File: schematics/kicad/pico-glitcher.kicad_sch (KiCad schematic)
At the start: 72 parts, among them Q1 IRLML2502, Q2 IRF7807PBF, Q3 TPS 79318, Q4 TPS2041, U1 NH245, U2 NH245, X1 BU-SMA-V, X2 BU-SMA, X3 M08X2

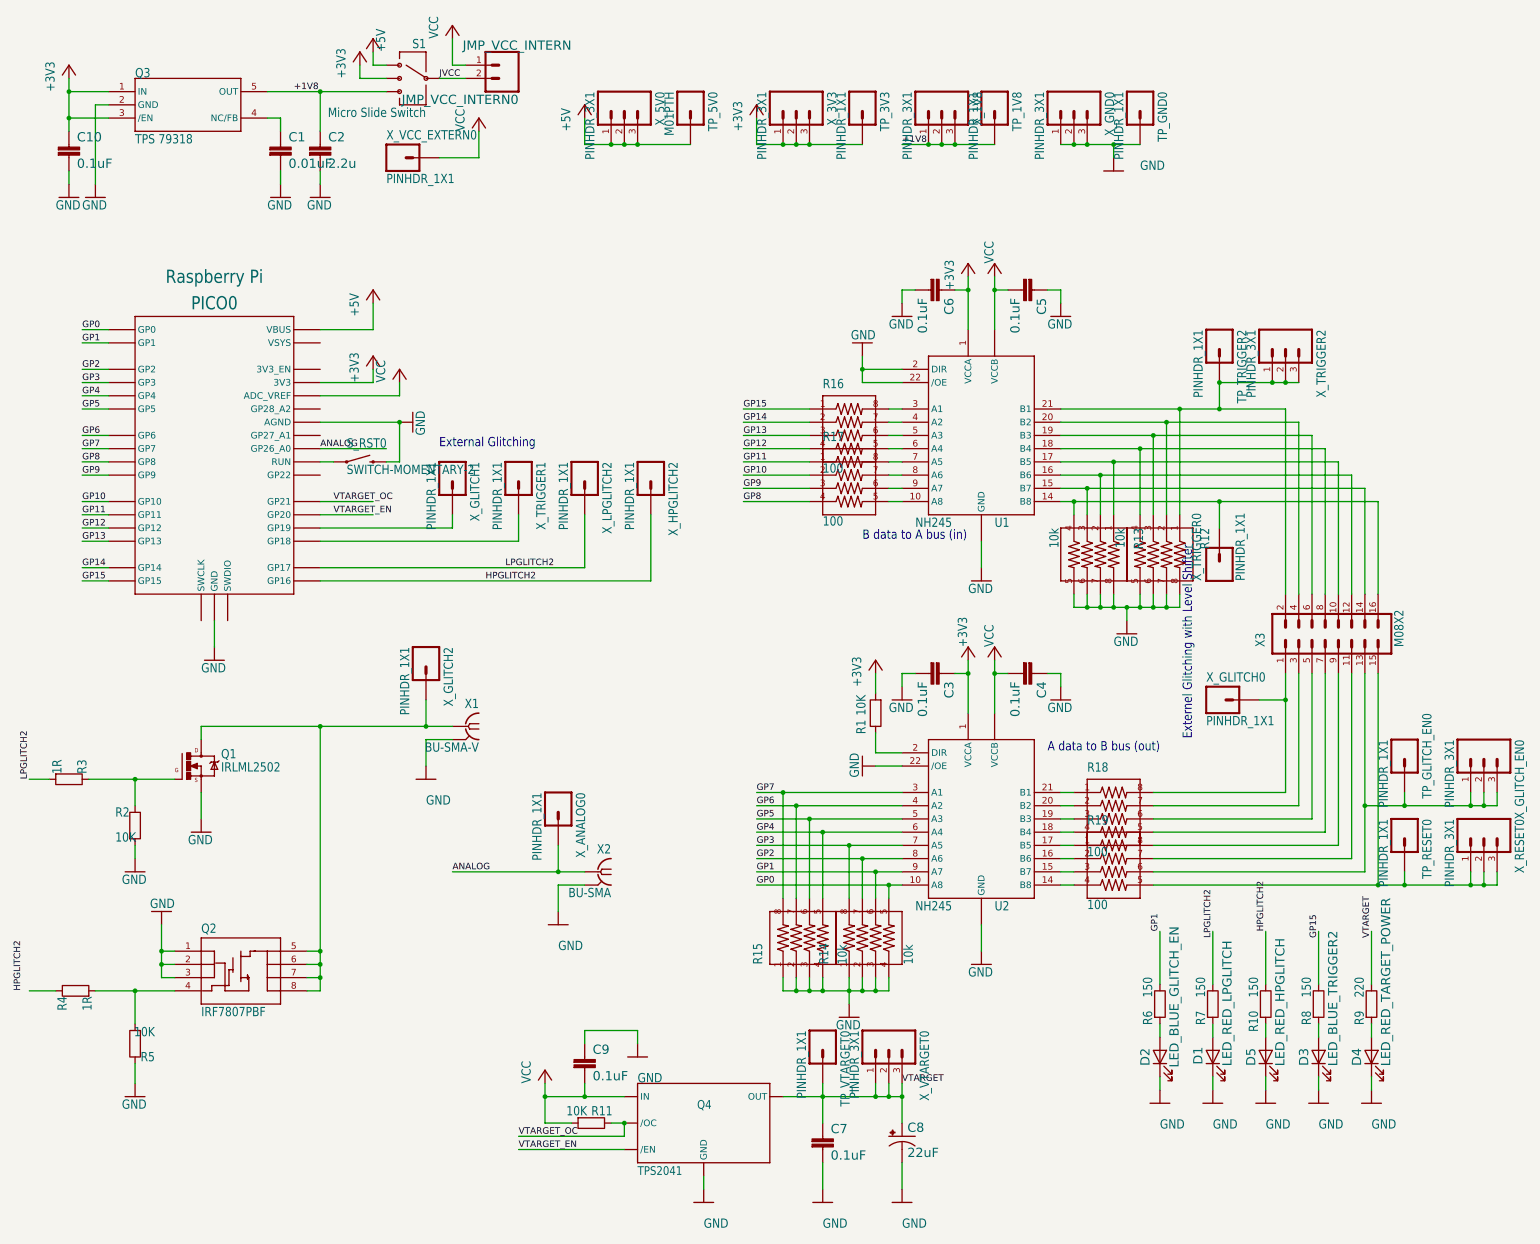
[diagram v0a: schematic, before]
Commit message: replaced 0603 capacitor's symbol and footprint with kicad library's ones
  also: simplified some tracks.
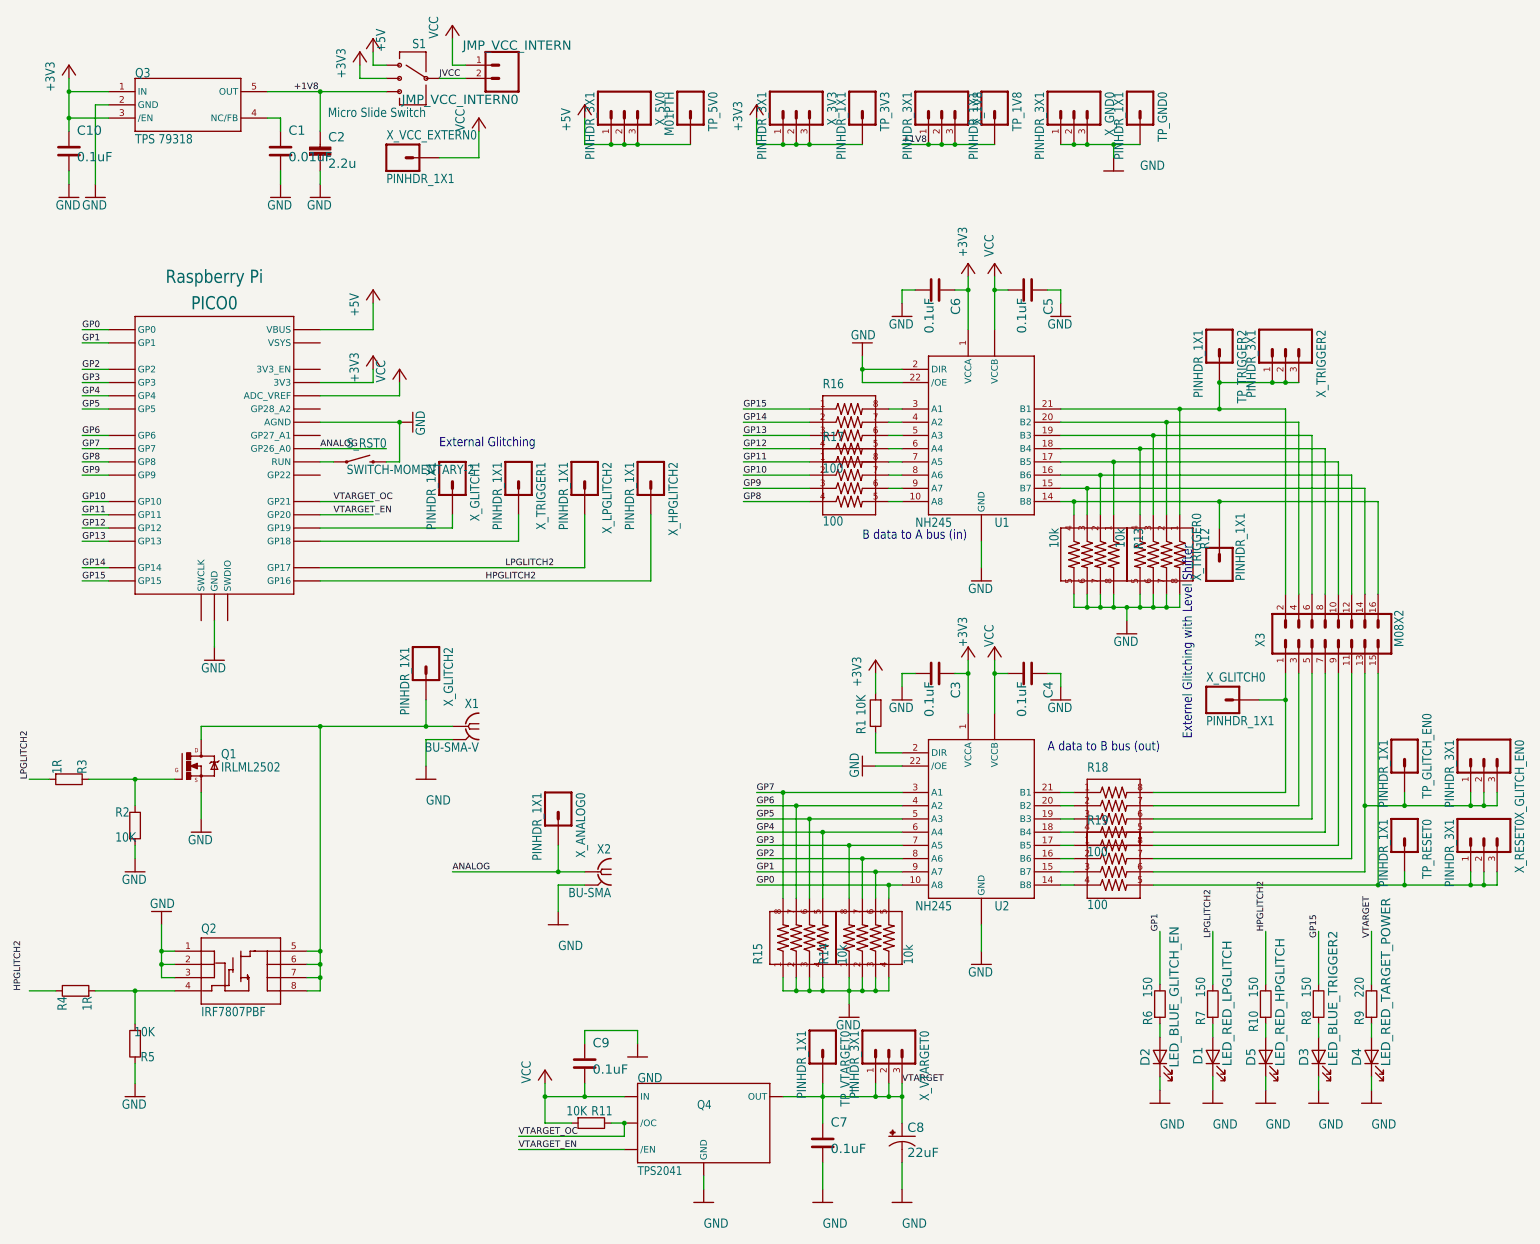
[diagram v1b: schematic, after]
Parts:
- C1, C10, C3, C4, C5, C6, C7, C9: footprint pico-glitcher:0603 -> Capacitor_SMD:C_0603_1608Metric; symbol pico-glitcher:0.1UF-0603-25V-10%-X7R-WE -> Device:C
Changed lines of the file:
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@@
 	)
 	(symbol
-		(lib_id "pico-glitcher:0.1UF-0603-25V-10%-X7R-WE")
-		(at 208.28 71.12 270)
+		(lib_id "Device:C")
+		(at 209.55 71.12 270)
 		(unit 1)
 		(exclude_from_sim no)
@@
 		(dnp no)
 		(property "Reference" "C5"
-			(at 211.201 72.644 0)
+			(at 212.471 72.644 0)
 			(effects
 				(font
@@
 		)
 		(property "Value" "0.1uF"
-			(at 206.121 72.644 0)
+			(at 207.391 72.644 0)
 			(effects
 				(font
@@
 			)
 		)
-		(property "Footprint" "pico-glitcher:0603"
-			(at 208.28 71.12 0)
+		(property "Footprint" "Capacitor_SMD:C_0603_1608Metric"
+			(at 205.74 72.0852 0)
 			(effects
 				(font
@@
 			)
 		)
-		(property "Datasheet" ""
-			(at 208.28 71.12 0)
+		(property "Datasheet" "~"
+			(at 209.55 71.12 0)
 			(effects
 				(font
@@
 			)
 		)
-		(property "Description" ""
-			(at 208.28 71.12 0)
+		(property "Description" "Unpolarized capacitor"
+			(at 209.55 71.12 0)
 			(effects
 				(font
@@
 	)
 	(symbol
-		(lib_id "pico-glitcher:0.1UF-0603-25V-10%-X7R-WE")
-		(at 190.5 71.12 270)
+		(lib_id "Device:C")
+		(at 191.77 71.12 270)
 		(unit 1)
 		(exclude_from_sim no)
@@
 		(dnp no)
 		(property "Reference" "C6"
-			(at 193.421 72.644 0)
+			(at 194.691 72.644 0)
 			(effects
 				(font
@@
 		)
 		(property "Value" "0.1uF"
-			(at 188.341 72.644 0)
+			(at 189.611 72.644 0)
 			(effects
 				(font
@@
 			)
 		)
-		(property "Footprint" "pico-glitcher:0603"
-			(at 190.5 71.12 0)
+		(property "Footprint" "Capacitor_SMD:C_0603_1608Metric"
+			(at 187.96 72.0852 0)
 			(effects
 				(font
@@
 			)
 		)
-		(property "Datasheet" ""
-			(at 190.5 71.12 0)
+		(property "Datasheet" "~"
+			(at 191.77 71.12 0)
 			(effects
 				(font
@@
 			)
 		)
-		(property "Description" ""
-			(at 190.5 71.12 0)
+		(property "Description" "Unpolarized capacitor"
+			(at 191.77 71.12 0)
 			(effects
 				(font
@@
 	)
 	(symbol
-		(lib_id "pico-glitcher:0.1UF-0603-25V-10%-X7R-WE")
-		(at 124.46 220.98 0)
+		(lib_id "Device:C")
+		(at 124.46 219.71 0)
 		(unit 1)
 		(exclude_from_sim no)
@@
 		(dnp no)
 		(property "Reference" "C9"
-			(at 125.984 218.059 0)
+			(at 125.984 216.789 0)
 			(effects
 				(font
@@
 		)
 		(property "Value" "0.1uF"
-			(at 125.984 223.139 0)
+			(at 125.984 221.869 0)
 			(effects
 				(font
@@
 			)
 		)
-		(property "Footprint" "pico-glitcher:0603"
-			(at 124.46 220.98 0)
+		(property "Footprint" "Capacitor_SMD:C_0603_1608Metric"
+			(at 125.4252 223.52 0)
 			(effects
 				(font
@@
 			)
 		)
-		(property "Datasheet" ""
-			(at 124.46 220.98 0)
+		(property "Datasheet" "~"
+			(at 124.46 219.71 0)
 			(effects
 				(font
@@
 			)
 		)
-		(property "Description" ""
-			(at 124.46 220.98 0)
+		(property "Description" "Unpolarized capacitor"
+			(at 124.46 219.71 0)
 			(effects
 				(font
@@
 	)
 	(symbol
-		(lib_id "pico-glitcher:0.1UF-0603-25V-10%-X7R-WE")
-		(at 208.28 144.78 270)
+		(lib_id "Device:C")
+		(at 209.55 144.78 270)
 		(unit 1)
 		(exclude_from_sim no)
@@
 		(dnp no)
 		(property "Reference" "C4"
-			(at 211.201 146.304 0)
+			(at 212.471 146.304 0)
 			(effects
 				(font
@@
 		)
 		(property "Value" "0.1uF"
-			(at 206.121 146.304 0)
+			(at 207.391 146.304 0)
 			(effects
 				(font
@@
 			)
 		)
-		(property "Footprint" "pico-glitcher:0603"
-			(at 208.28 144.78 0)
+		(property "Footprint" "Capacitor_SMD:C_0603_1608Metric"
+			(at 205.74 145.7452 0)
 			(effects
 				(font
@@
 			)
 		)
-		(property "Datasheet" ""
-			(at 208.28 144.78 0)
+		(property "Datasheet" "~"
+			(at 209.55 144.78 0)
 			(effects
 				(font
@@
 			)
 		)
-		(property "Description" ""
-			(at 208.28 144.78 0)
+		(property "Description" "Unpolarized capacitor"
+			(at 209.55 144.78 0)
 			(effects
 				(font
@@
 	)
 	(symbol
-		(lib_id "pico-glitcher:0.1UF-0603-25V-10%-X7R-WE")
-		(at 66.04 45.72 0)
+		(lib_id "Device:C")
+		(at 66.04 44.45 0)
 		(unit 1)
 		(exclude_from_sim no)
@@
 		(dnp no)
 		(property "Reference" "C1"
-			(at 67.564 42.799 0)
+			(at 67.564 41.529 0)
 			(effects
 				(font
@@
 		)
 		(property "Value" "0.01uF"
-			(at 67.564 47.879 0)
+			(at 67.564 46.609 0)
 			(effects
 				(font
@@
 			)
 		)
-		(property "Footprint" "pico-glitcher:0603"
-			(at 66.04 45.72 0)
+		(property "Footprint" "Capacitor_SMD:C_0603_1608Metric"
+			(at 67.0052 48.26 0)
 			(effects
 				(font
@@
 			)
 		)
-		(property "Datasheet" ""
-			(at 66.04 45.72 0)
+		(property "Datasheet" "~"
+			(at 66.04 44.45 0)
 			(effects
 				(font
@@
 			)
 		)
-		(property "Description" ""
-			(at 66.04 45.72 0)
+		(property "Description" "Unpolarized capacitor"
+			(at 66.04 44.45 0)
 			(effects
 				(font
@@
 	)
 	(symbol
-		(lib_id "pico-glitcher:0.1UF-0603-25V-10%-X7R-WE")
-		(at 170.18 236.22 0)
+		(lib_id "Device:C")
+		(at 170.18 234.95 0)
 		(unit 1)
 		(exclude_from_sim no)
@@
 		(dnp no)
 		(property "Reference" "C7"
-			(at 171.704 233.299 0)
+			(at 171.704 232.029 0)
 			(effects
 				(font
@@
 		)
 		(property "Value" "0.1uF"
-			(at 171.704 238.379 0)
+			(at 171.704 237.109 0)
 			(effects
 				(font
@@
 			)
 		)
-		(property "Footprint" "pico-glitcher:0603"
-			(at 170.18 236.22 0)
+		(property "Footprint" "Capacitor_SMD:C_0603_1608Metric"
+			(at 171.1452 238.76 0)
 			(effects
 				(font
@@
 			)
 		)
-		(property "Datasheet" ""
-			(at 170.18 236.22 0)
+		(property "Datasheet" "~"
+			(at 170.18 234.95 0)
 			(effects
 				(font
@@
 			)
 		)
-		(property "Description" ""
-			(at 170.18 236.22 0)
+		(property "Description" "Unpolarized capacitor"
+			(at 170.18 234.95 0)
 			(effects
 				(font
@@
 		)
 		(property "Value" "VCC"
-			(at 203.2 66.04 90)
+			(at 203.2 64.77 90)
 			(effects
 				(font
@@
 	)
 	(symbol
-		(lib_id "pico-glitcher:0.1UF-0603-25V-10%-X7R-WE")
-		(at 25.4 45.72 0)
+		(lib_id "Device:C")
+		(at 25.4 44.45 0)
 		(unit 1)
 		(exclude_from_sim no)
@@
 		(dnp no)
 		(property "Reference" "C10"
-			(at 26.924 42.799 0)
+			(at 26.924 41.529 0)
 			(effects
 				(font
@@
 		)
 		(property "Value" "0.1uF"
-			(at 26.924 47.879 0)
+			(at 26.924 46.609 0)
 			(effects
 				(font
@@
 			)
 		)
-		(property "Footprint" "pico-glitcher:0603"
-			(at 25.4 45.72 0)
+		(property "Footprint" "Capacitor_SMD:C_0603_1608Metric"
+			(at 26.3652 48.26 0)
 			(effects
 				(font
@@
 			)
 		)
-		(property "Datasheet" ""
-			(at 25.4 45.72 0)
+		(property "Datasheet" "~"
+			(at 25.4 44.45 0)
 			(effects
 				(font
@@
 			)
 		)
-		(property "Description" ""
-			(at 25.4 45.72 0)
+		(property "Description" "Unpolarized capacitor"
+			(at 25.4 44.45 0)
 			(effects
 				(font
@@
 		)
 		(property "Value" "+3V3"
-			(at 195.58 71.12 90)
+			(at 198.12 64.77 90)
 			(effects
 				(font
@@
 	)
 	(symbol
-		(lib_id "pico-glitcher:0.1UF-0603-25V-10%-X7R-WE")
-		(at 190.5 144.78 270)
+		(lib_id "Device:C")
+		(at 191.77 144.78 270)
 		(unit 1)
 		(exclude_from_sim no)
@@
 		(dnp no)
 		(property "Reference" "C3"
-			(at 193.421 146.304 0)
+			(at 194.691 146.304 0)
 			(effects
 				(font
@@
 		)
 		(property "Value" "0.1uF"
-			(at 188.341 146.304 0)
+			(at 189.611 146.304 0)
 			(effects
 				(font
@@
 			)
 		)
-		(property "Footprint" "pico-glitcher:0603"
-			(at 190.5 144.78 0)
+		(property "Footprint" "Capacitor_SMD:C_0603_1608Metric"
+			(at 187.96 145.7452 0)
 			(effects
 				(font
@@
 			)
 		)
-		(property "Datasheet" ""
-			(at 190.5 144.78 0)
+		(property "Datasheet" "~"
+			(at 191.77 144.78 0)
 			(effects
 				(font
@@
 			)
 		)
-		(property "Description" ""
-			(at 190.5 144.78 0)
+		(property "Description" "Unpolarized capacitor"
+			(at 191.77 144.78 0)
 			(effects
 				(font
